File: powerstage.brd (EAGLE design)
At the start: 42 x 43.5 mm, 40 parts, among them CON1 PINHEAD_1X10-2-FEMALE, CON2 BATTERY_CON-2P-XT30-RA, CON3 PINHEAD_1X10-2-FEMALE, IC5 MCP9700, Q1 BUK7K6R2-40EX, Q2 BUK7K6R2-40EX, Q3 BUK7K6R2-40EX

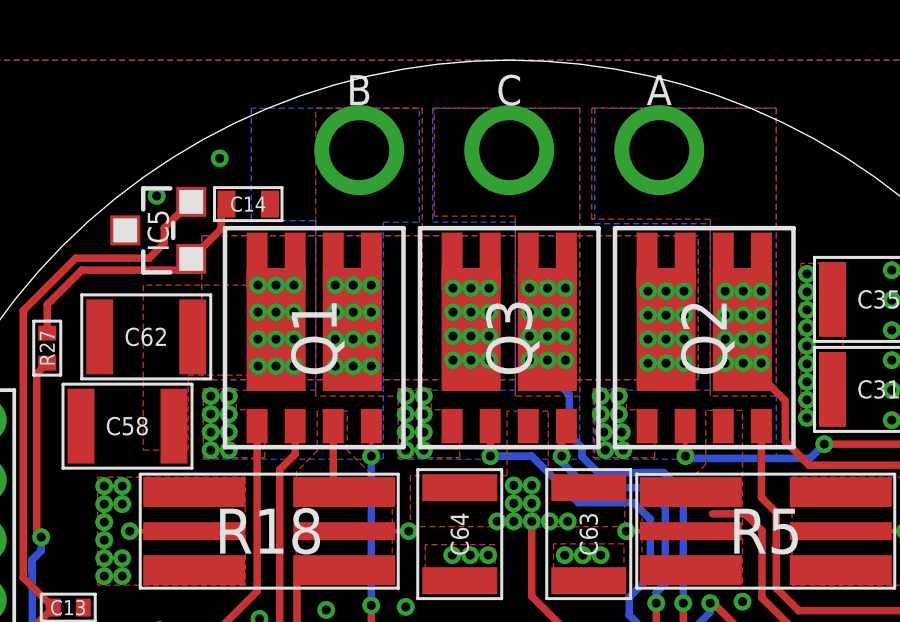
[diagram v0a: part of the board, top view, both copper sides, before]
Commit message: powerstage updates
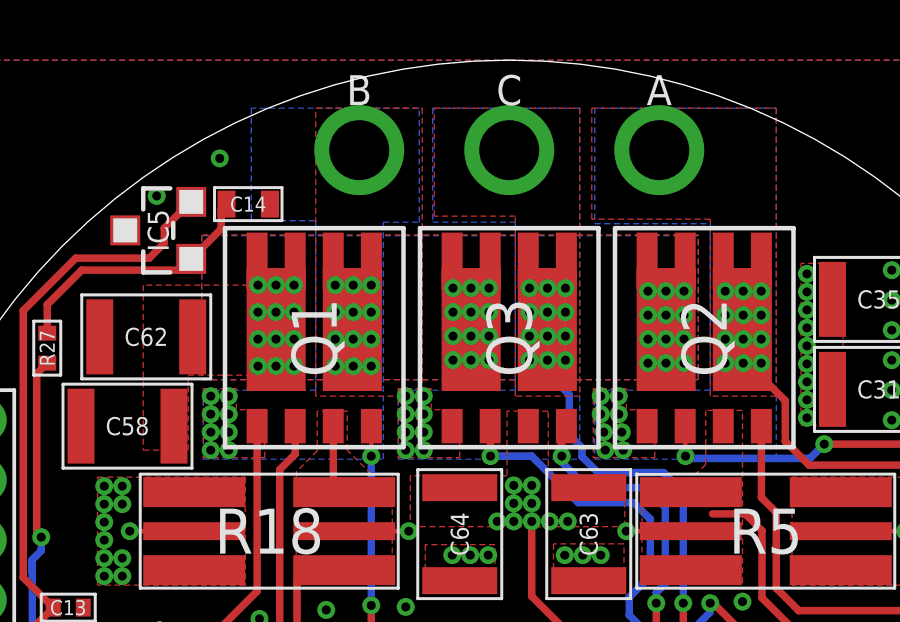
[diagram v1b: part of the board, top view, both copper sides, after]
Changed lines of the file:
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@@
 <setting verticaltext="up"/>
 </settings>
-<grid distance="0.05" unitdist="mm" unit="mm" style="lines" multiple="2" display="yes" altdistance="5" altunitdist="mil" altunit="mil"/>
+<grid distance="0.025" unitdist="mm" unit="mm" style="lines" multiple="2" display="yes" altdistance="5" altunitdist="mil" altunit="mil"/>
 <layers>
 <layer number="1" name="Top" color="4" fill="1" visible="yes" active="yes"/>
@@
 <layer number="25" name="tNames" color="7" fill="1" visible="yes" active="yes"/>
 <layer number="26" name="bNames" color="7" fill="1" visible="no" active="yes"/>
-<layer number="27" name="tValues" color="7" fill="1" visible="no" active="yes"/>
+<layer number="27" name="tValues" color="7" fill="1" visible="yes" active="yes"/>
 <layer number="28" name="bValues" color="7" fill="1" visible="no" active="yes"/>
 <layer number="29" name="tStop" color="7" fill="3" visible="no" active="yes"/>
@@
 <vertex x="6.3" y="10.35"/>
 </polygon>
-<polygon width="0.1524" layer="1" thermals="no" rank="3">
-<vertex x="6.3" y="15.15"/>
-<vertex x="-10.25" y="15.15"/>
+<polygon width="0.1524" layer="1" thermals="no" rank="4">
+<vertex x="6.3" y="15.175"/>
+<vertex x="-10.25" y="15.175"/>
 <vertex x="-10.25" y="10.35"/>
 <vertex x="6.3" y="10.35"/>
@@
 <contactref element="Q3" pad="5" route="any" routetag="T2.D"/>
 <contactref element="Q3" pad="1"/>
-<polygon width="0.1524" layer="1" thermals="no" rank="2">
+<polygon width="0.1524" layer="1" thermals="no" rank="3">
 <vertex x="0.2" y="9.8"/>
 <vertex x="0.2" y="15.8"/>
@@
 <contactref element="Q1" pad="1"/>
 <contactref element="B" pad="P$1"/>
-<polygon width="0.1524" layer="1" thermals="no">
+<polygon width="0.1524" layer="1" thermals="no" rank="2">
 <vertex x="-6.45" y="9.8"/>
 <vertex x="-6.45" y="19.4"/>
